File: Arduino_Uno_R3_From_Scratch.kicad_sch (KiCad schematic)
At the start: 0 parts

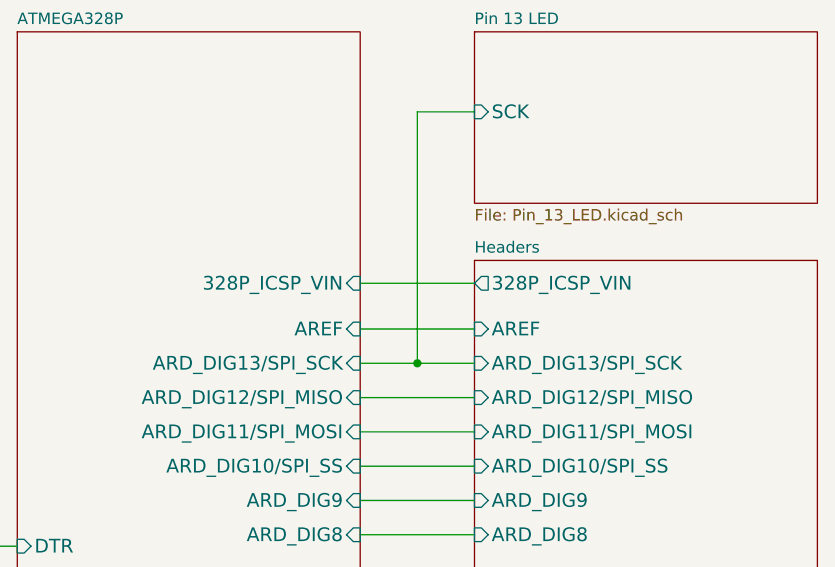
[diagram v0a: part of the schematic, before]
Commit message: update power symbols
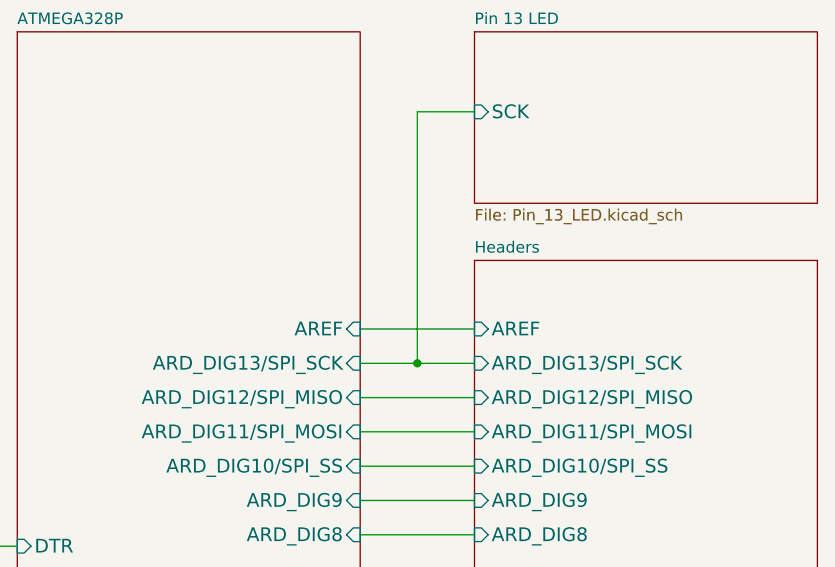
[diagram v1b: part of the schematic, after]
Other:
- sheet ATMEGA328P ports: added none; removed 328P_ICSP_VIN
- sheet Headers ports: added none; removed 328P_ICSP_VIN
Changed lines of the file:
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@@
-    (stroke (width 0) (type default))
-  )
-  (wire (pts (xy 179.07 63.5) (xy 191.77 63.5))
     (stroke (width 0) (type default))
   )
@@
       (effects (font (size 1.524 1.524)) (justify right))
     )
-    (pin "328P_ICSP_VIN" input (at 179.07 63.5 0)
-      (effects (font (size 1.524 1.524)) (justify right))
-    )
     (instances
       (project "Arduino_Uno_R3_From_Scratch"
@@
       (effects (font (size 1.524 1.524)) (justify left))
     )
-    (pin "328P_ICSP_VIN" output (at 191.77 63.5 180)
-      (effects (font (size 1.524 1.524)) (justify left))
-    )

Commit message: change power symbols and Arduino header
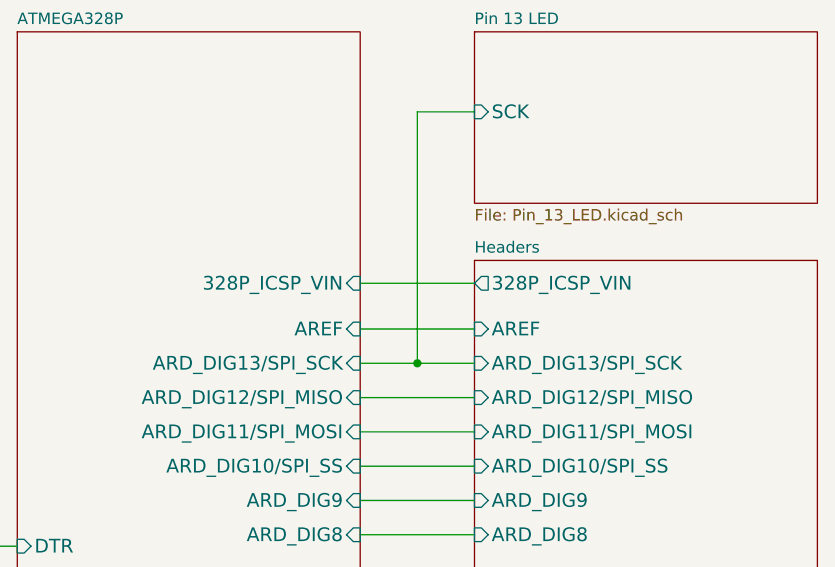
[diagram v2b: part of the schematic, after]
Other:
- sheet ATMEGA328P ports: added 328P_ICSP_VIN; removed none
- sheet Headers ports: added 328P_ICSP_VIN; removed none
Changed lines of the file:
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@@
+    (stroke (width 0) (type default))
+  )
+  (wire (pts (xy 179.07 63.5) (xy 191.77 63.5))
     (stroke (width 0) (type default))
   )
@@
       (effects (font (size 1.524 1.524)) (justify right))
     )
+    (pin "328P_ICSP_VIN" input (at 179.07 63.5 0)
+      (effects (font (size 1.524 1.524)) (justify right))
+    )
     (instances
       (project "Arduino_Uno_R3_From_Scratch"
@@
       (effects (font (size 1.524 1.524)) (justify left))
     )
+    (pin "328P_ICSP_VIN" output (at 191.77 63.5 180)
+      (effects (font (size 1.524 1.524)) (justify left))
+    )
